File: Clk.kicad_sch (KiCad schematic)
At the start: 14 parts, among them U30 74LVC1G125GW, U5 SiT2001, U6 74LVC1G74DC, U7 74LVC1G74DC

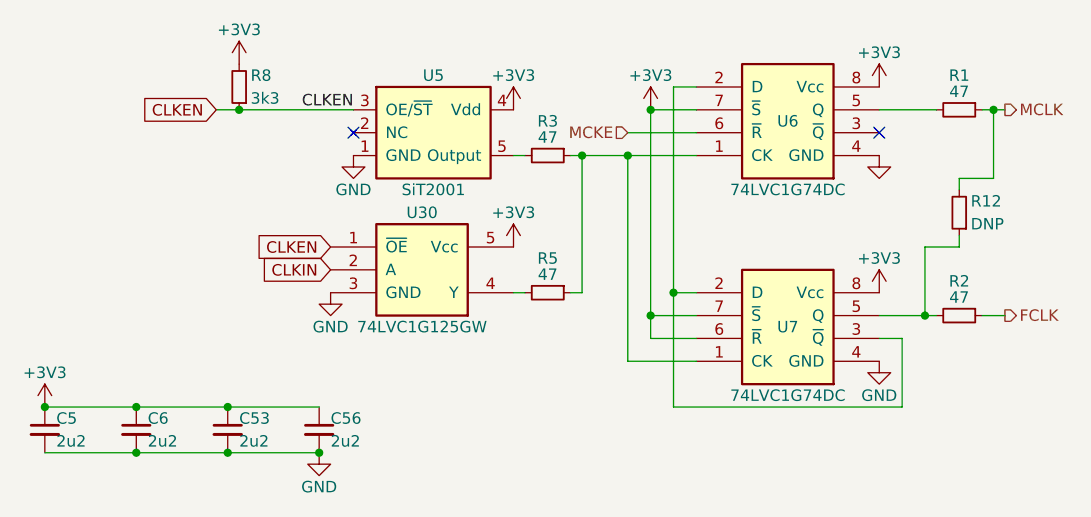
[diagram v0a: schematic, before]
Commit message: Final A?
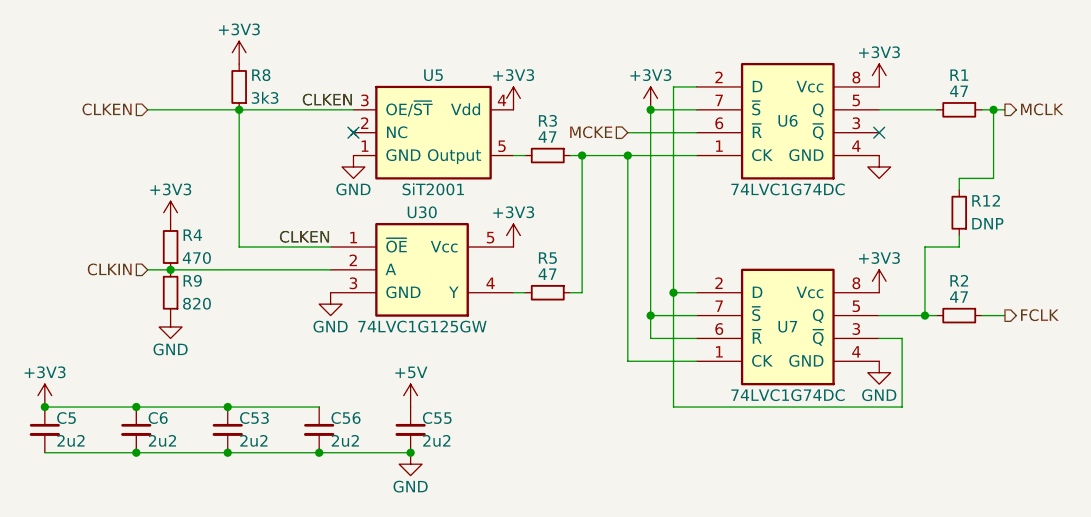
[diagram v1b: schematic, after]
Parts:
- added C55: 2u2, stdpads:C_0603, symbol Device:C_Small
- added R4: 470, stdpads:R_0603, symbol Device:R_Small
- added R9: 820, stdpads:R_0603, symbol Device:R_Small
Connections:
- net +3V3: now also R4.2
- net CLKIN: now also R4.1, R9.2
- net GND: now also C55.2, R9.1
- new net +5V: C55.1
